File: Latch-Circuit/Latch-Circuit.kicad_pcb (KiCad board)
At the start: 4 copper layers, 50 x 40 mm, 67 parts, among them J1 2-1445052-2, J2 3-794633-8, J3 B2P-VH, J4 3-794633-6, Q1 DMP3098LQ-7, Q2 2N7002K-AU_R1_000A2, Q3 2N7002K-AU_R1_000A2, Q4 2N7002K-AU_R1_000A2, U1 TLP3106A(TP,F, U2 TLP3106A(TP,F, U3 TLP3106A(TP,F, U4 CD4043BPWR, U5 TBD62003AFNG,EL

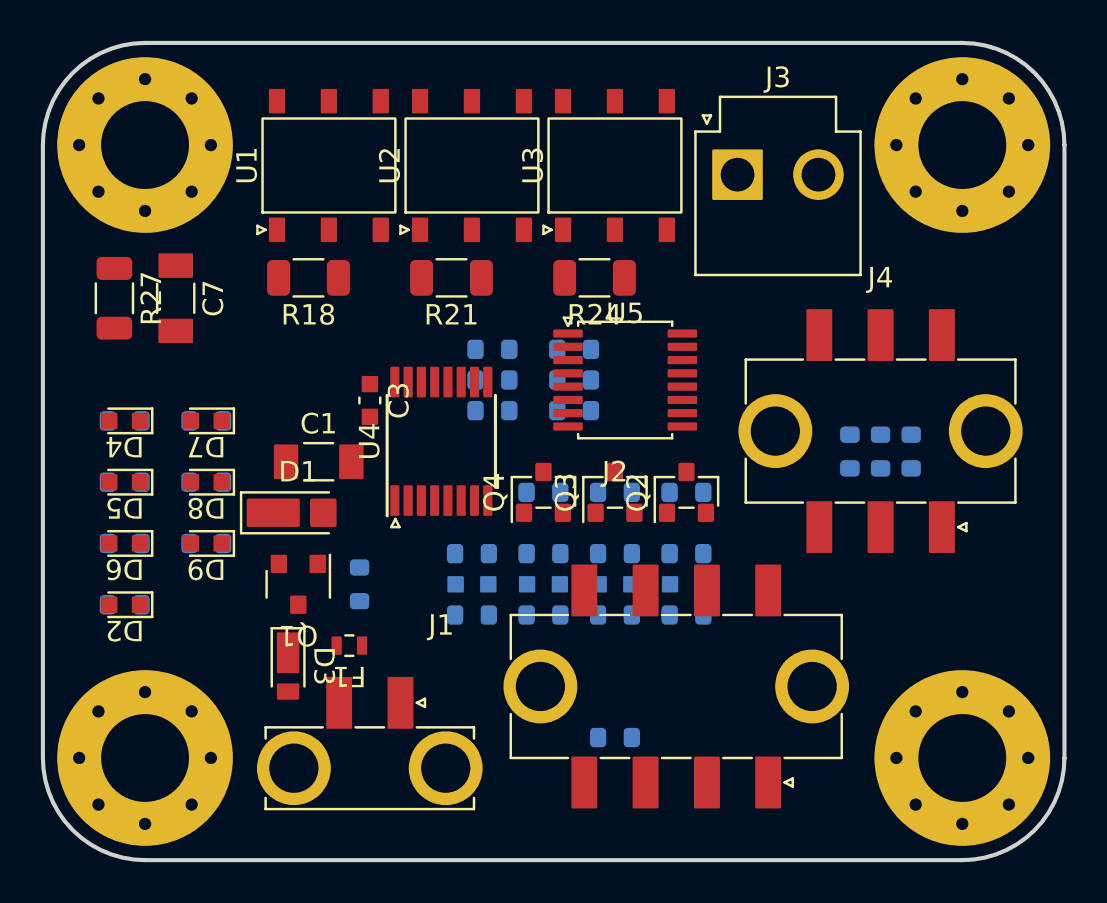
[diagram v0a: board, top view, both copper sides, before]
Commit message: finish wiring
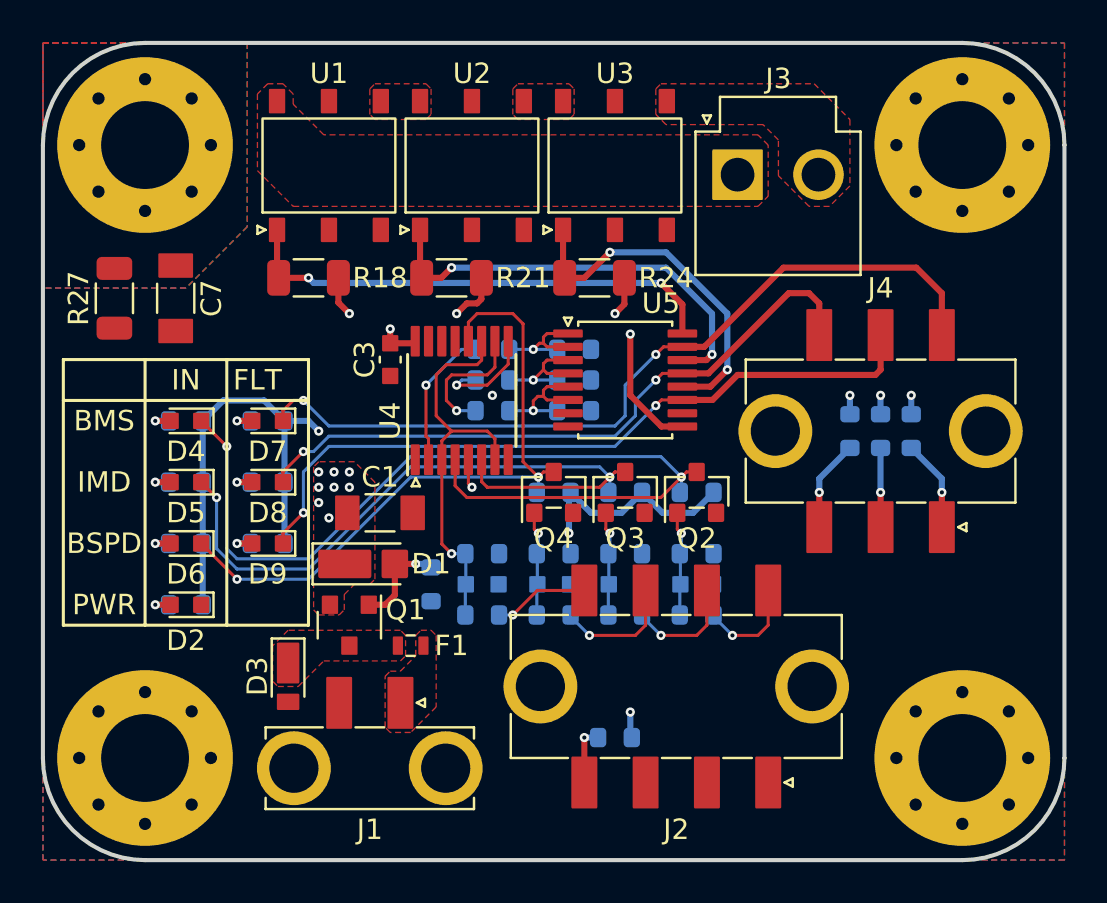
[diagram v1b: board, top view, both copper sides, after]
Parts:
- moved D1 4.30 mm to (16.0, 25.5)
- moved C1 3.91 mm to (16.5, 23.0)
- moved R1 3.50 mm to (19.0, 26.5)
- moved Q1 3.20 mm to (15.0, 28.5)
- moved D2 3.00 mm to (7.00, 27.5)
- moved D4 3.00 mm to (7.00, 18.5)
- moved D5 3.00 mm to (7.00, 21.5)
- moved D6 3.00 mm to (7.00, 24.5)
- moved D7 3.00 mm to (11.0, 18.5)
- moved D8 3.00 mm to (11.0, 21.5)
- moved D9 3.00 mm to (11.0, 24.5)
- moved F1 3.00 mm to (18.0, 29.5)
- moved R2 3.00 mm to (7.00, 27.5)
- moved R28 3.00 mm to (11.0, 18.5)
- moved R29 3.00 mm to (11.0, 21.5)
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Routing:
- net +12V: track 0.00 -> 53.5 mm, vias 0 -> 20
- net ~{BMS_STATUS}: track 0.00 -> 46.3 mm, vias 0 -> 2
- net BMS_LED_K: track 0.00 -> 40.1 mm, vias 0 -> 2
- net BSPD_LED_K: track 0.00 -> 35.9 mm, vias 0 -> 2
- net ~{IMD_STATUS}: track 0.00 -> 34.8 mm, vias 0 -> 2
- net ~{BSPD_STATUS}: track 0.00 -> 32.7 mm, vias 0 -> 2
- net IMD_LED_K: track 0.00 -> 32.6 mm, vias 0 -> 2
- net BMS_RLY_OFF: track 0.00 -> 24.1 mm, vias 0 -> 2
- net IMD_RLY_OFF: track 0.00 -> 21.3 mm, vias 0 -> 2
- net RST: track 0.00 -> 19.9 mm, vias 0 -> 1
- net BSPD_RLY_OFF: track 0.00 -> 17.4 mm, vias 0 -> 2
- net BMS_FAULT: track 0.00 -> 6.85 mm, vias 0 -> 1
- net BSPD_FAULT: track 0.00 -> 6.54 mm, vias 0 -> 1
- net Net-(U5-I5): track 0.00 -> 6.26 mm, vias 0 -> 1
- net BSPD_STATUS: track 0.00 -> 6.04 mm, vias 0 -> 1
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- added copper zone on F.Cu, net +12V
- added copper zone on In2.Cu, net +12V
- added copper zone on F.Cu, net /GLV_IN
- added copper zone on F.Cu, net /SHDN_IN
- added copper zone on F.Cu, net /SHDN_OUT
- added copper zone on B.Cu, net Chassis
- added copper zone on F.Cu, net Chassis
- added copper zone on In1.Cu, net Chassis
- added copper zone on In2.Cu, net Chassis
- added copper zone on B.Cu, net GND
- added copper zone on F.Cu, net GND
- added copper zone on In1.Cu, net GND
- added copper zone on In2.Cu, net GND
- added copper zone on F.Cu, net Net-(D3-K)
- added copper zone on F.Cu, net Net-(U1-Drain-Pad4)
- added copper zone on F.Cu, net Net-(U2-Drain-Pad4)
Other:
- board text added: "BMS"
- board text added: "BSPD"
- board text added: "FLT"
- board text added: "IMD"
- board text added: "IN"
- board text added: "PWR"
